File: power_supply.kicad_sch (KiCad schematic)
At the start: 17 parts

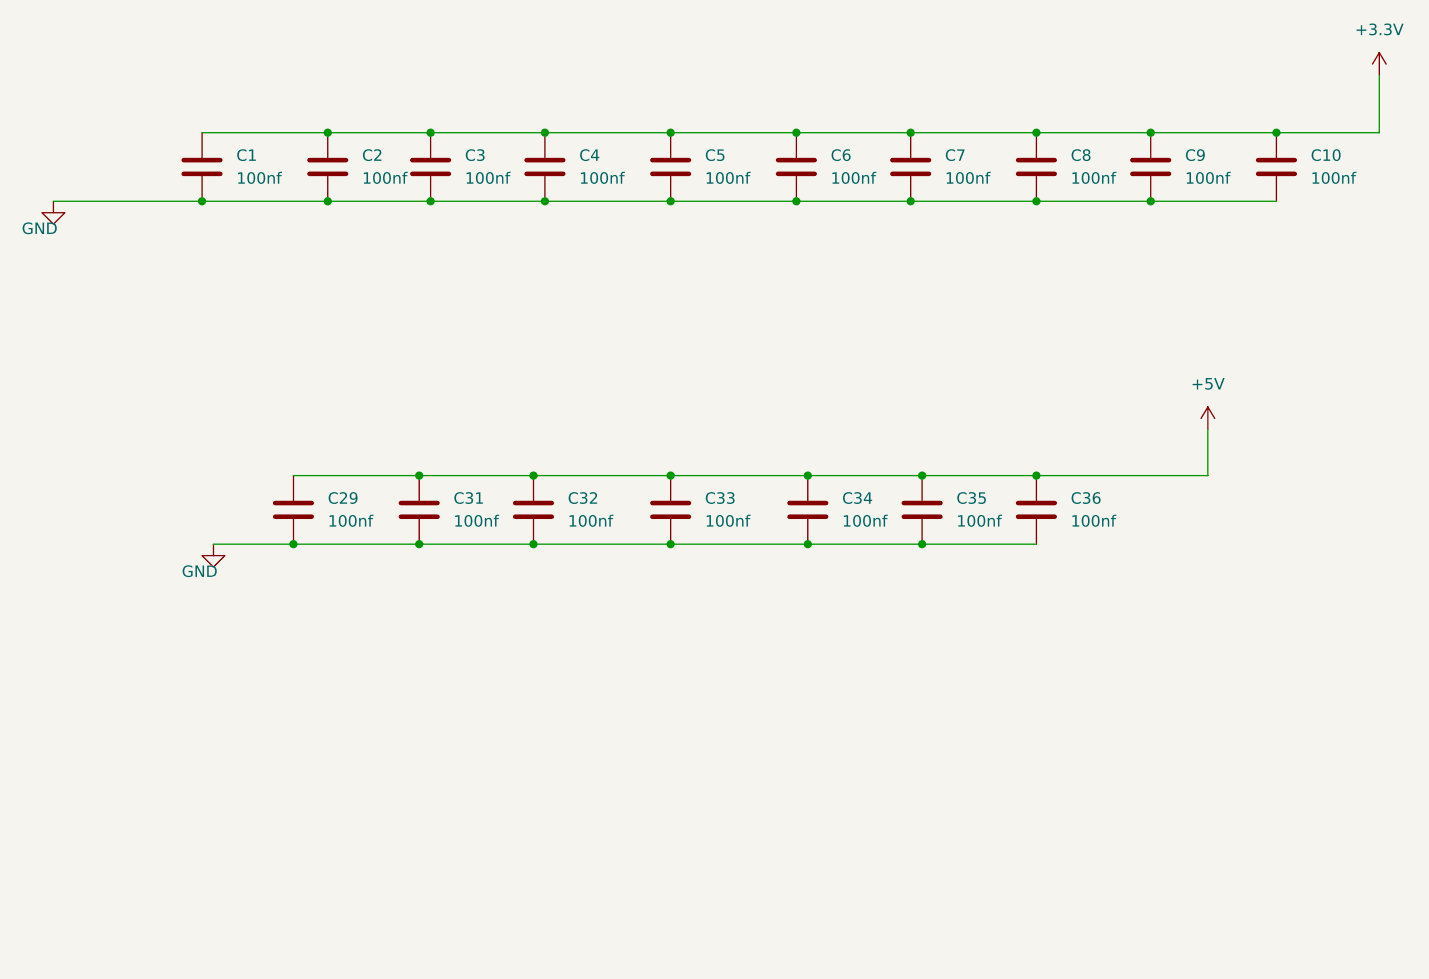
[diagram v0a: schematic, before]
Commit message: ESP32S3 branch initial changes
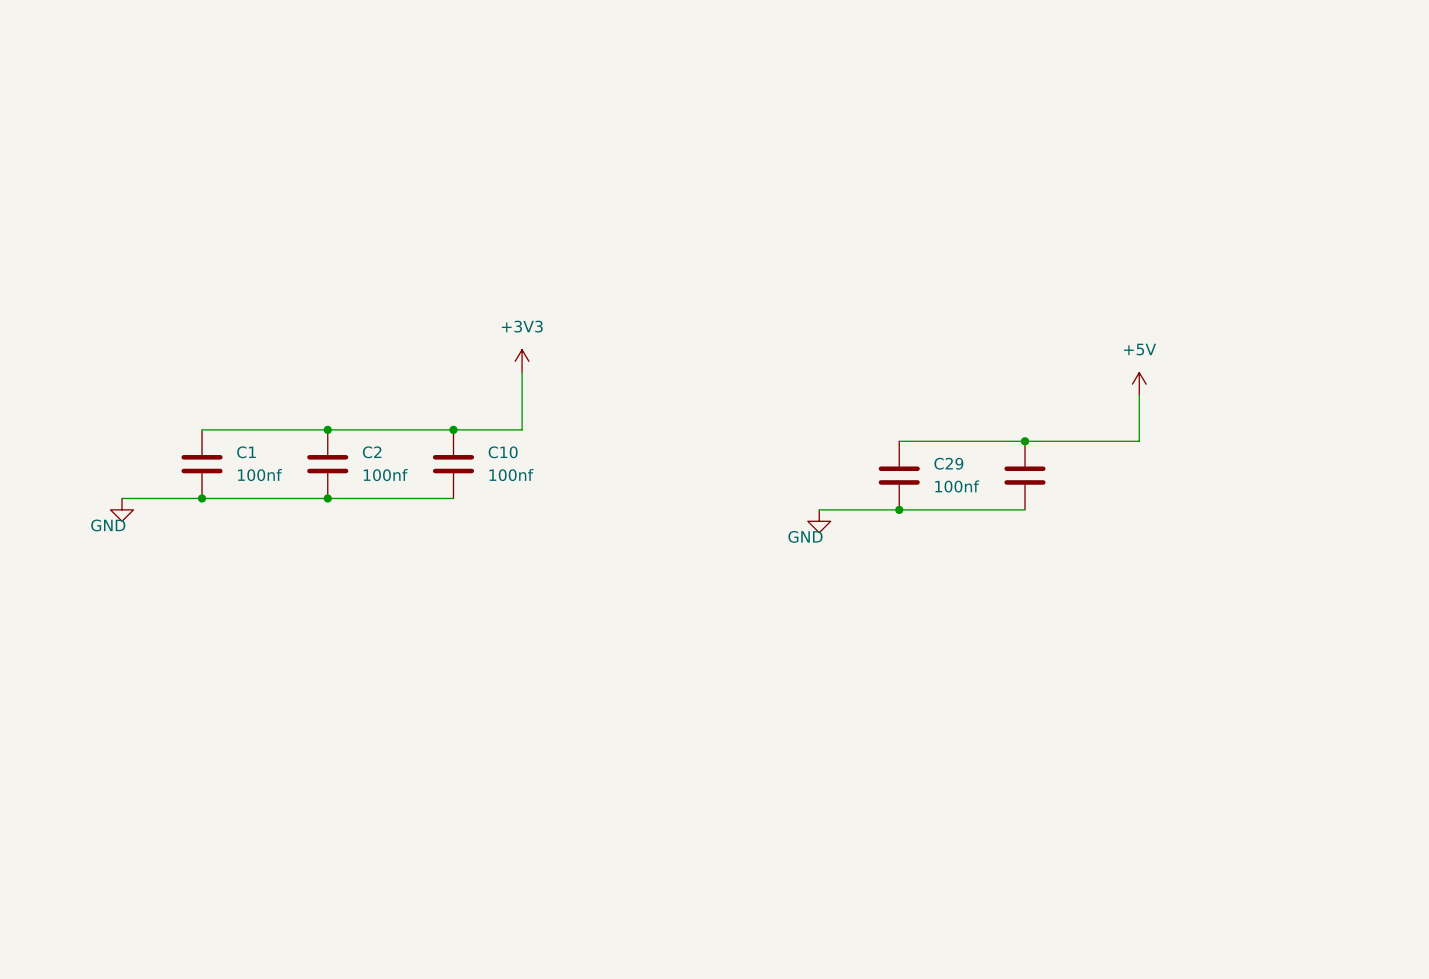
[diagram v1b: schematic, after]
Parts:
- removed C3, C32, C33, C34, C35, C36, C4, C5, C6, C7, C8, C9: 100nf, Capacitor_SMD:C_0805_2012Metric, symbol Device:C
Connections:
- net +3.3V renamed +3V3
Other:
- moved on the sheet: C1, C10, C2, C29

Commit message: Update KiCad project files
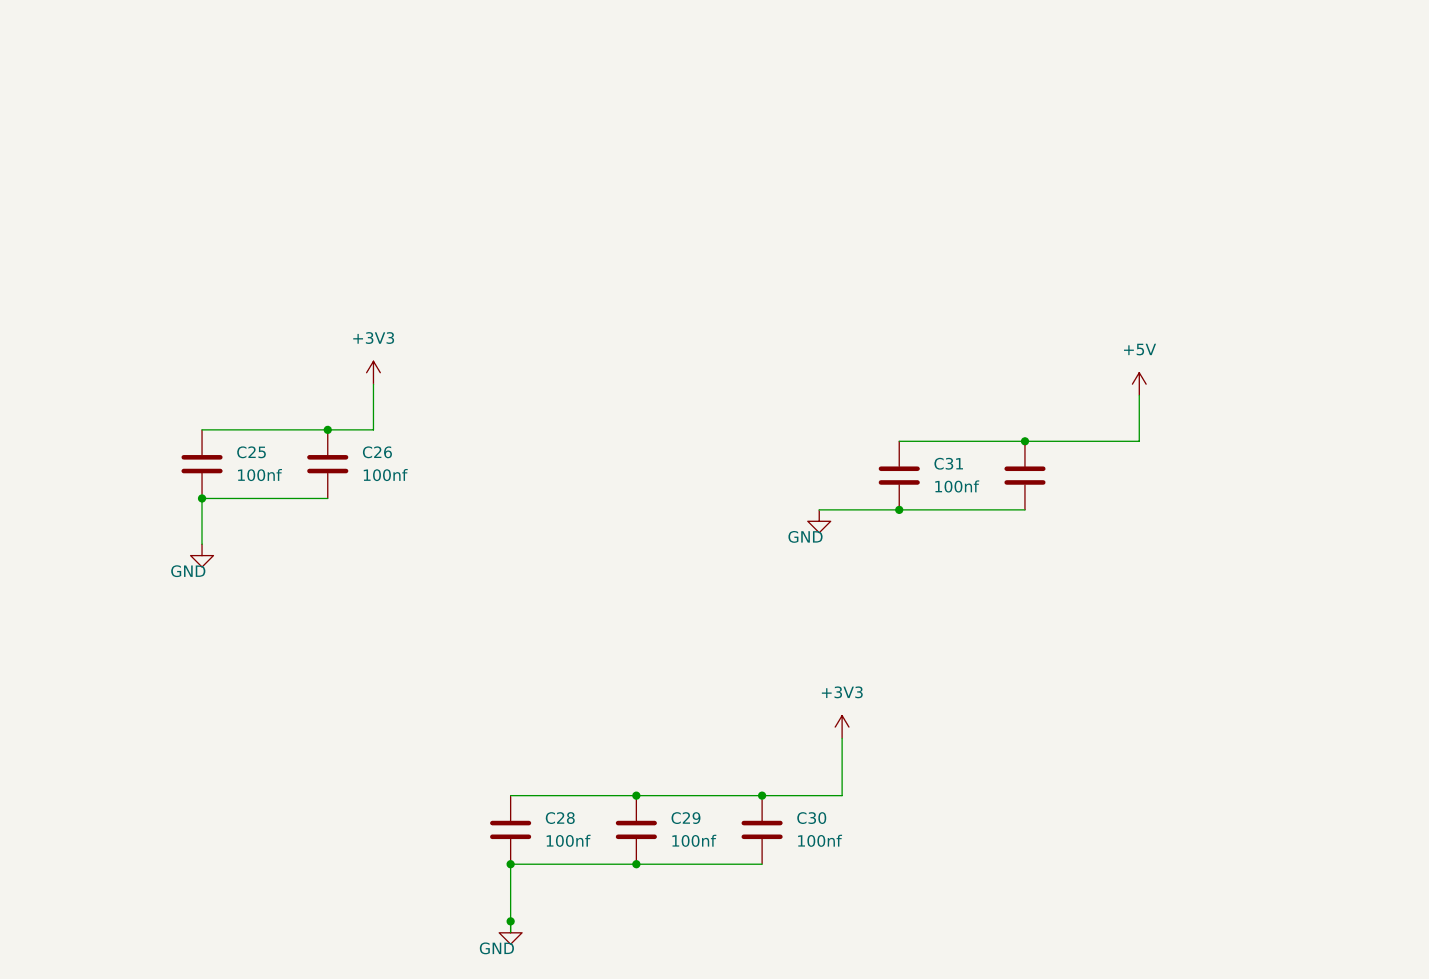
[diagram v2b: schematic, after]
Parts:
- removed C10: 100nf, Capacitor_SMD:C_0805_2012Metric, symbol Device:C
- added C28, C29, C30: 100nf, Capacitor_SMD:C_0805_2012Metric, symbol Device:C
- renumbered C1 to C25, C2 to C26, C29 to C31, C31 to C32
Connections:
- net +3V3: now also C28.1, C29.1, C30.1
- net GND: now also C28.2, C29.2, C30.2

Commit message: Remove unused schematic files, lock files, and backup directories
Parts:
- C25, C26, C28, C29, C30, C31, C32: footprint Capacitor_SMD:C_0805_2012Metric -> Capacitor_SMD:C_1206_3216Metric
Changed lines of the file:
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@@
 			)
 		)
-		(property "Footprint" "Capacitor_SMD:C_0805_2012Metric"
+		(property "Footprint" "Capacitor_SMD:C_1206_3216Metric"
 			(at 124.1552 134.62 0)
 			(hide yes)
@@
 			)
 		)
-		(property "Footprint" "Capacitor_SMD:C_0805_2012Metric"
+		(property "Footprint" "Capacitor_SMD:C_1206_3216Metric"
 			(at 138.1252 134.62 0)
 			(hide yes)
@@
 			)
 		)
-		(property "Footprint" "Capacitor_SMD:C_0805_2012Metric"
+		(property "Footprint" "Capacitor_SMD:C_1206_3216Metric"
 			(at 167.3352 95.25 0)
 			(hide yes)
@@
 			)
 		)
-		(property "Footprint" "Capacitor_SMD:C_0805_2012Metric"
+		(property "Footprint" "Capacitor_SMD:C_1206_3216Metric"
 			(at 152.0952 134.62 0)
 			(hide yes)
@@
 			)
 		)
-		(property "Footprint" "Capacitor_SMD:C_0805_2012Metric"
+		(property "Footprint" "Capacitor_SMD:C_1206_3216Metric"
 			(at 103.8352 93.98 0)
 			(hide yes)
@@
 			)
 		)
-		(property "Footprint" "Capacitor_SMD:C_0805_2012Metric"
+		(property "Footprint" "Capacitor_SMD:C_1206_3216Metric"
 			(at 181.3052 95.25 0)
 			(hide yes)
@@
 			)
 		)
-		(property "Footprint" "Capacitor_SMD:C_0805_2012Metric"
+		(property "Footprint" "Capacitor_SMD:C_1206_3216Metric"
 			(at 89.8652 93.98 0)
 			(hide yes)
